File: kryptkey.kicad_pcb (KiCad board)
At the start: 2 copper layers, 30 x 36.1 mm, 36 parts, among them J1 Conn_01x04_Pin, J2 Conn_01x04_Pin, J3 USB4155-03-C_REVA, SW1 SW_Push, SW2 SW_Push, SW3 SW_Push, SW4 SW_SPDT, U1 AMS1117-3.3, U2 STM32F103C8T6, Y1 16MHz

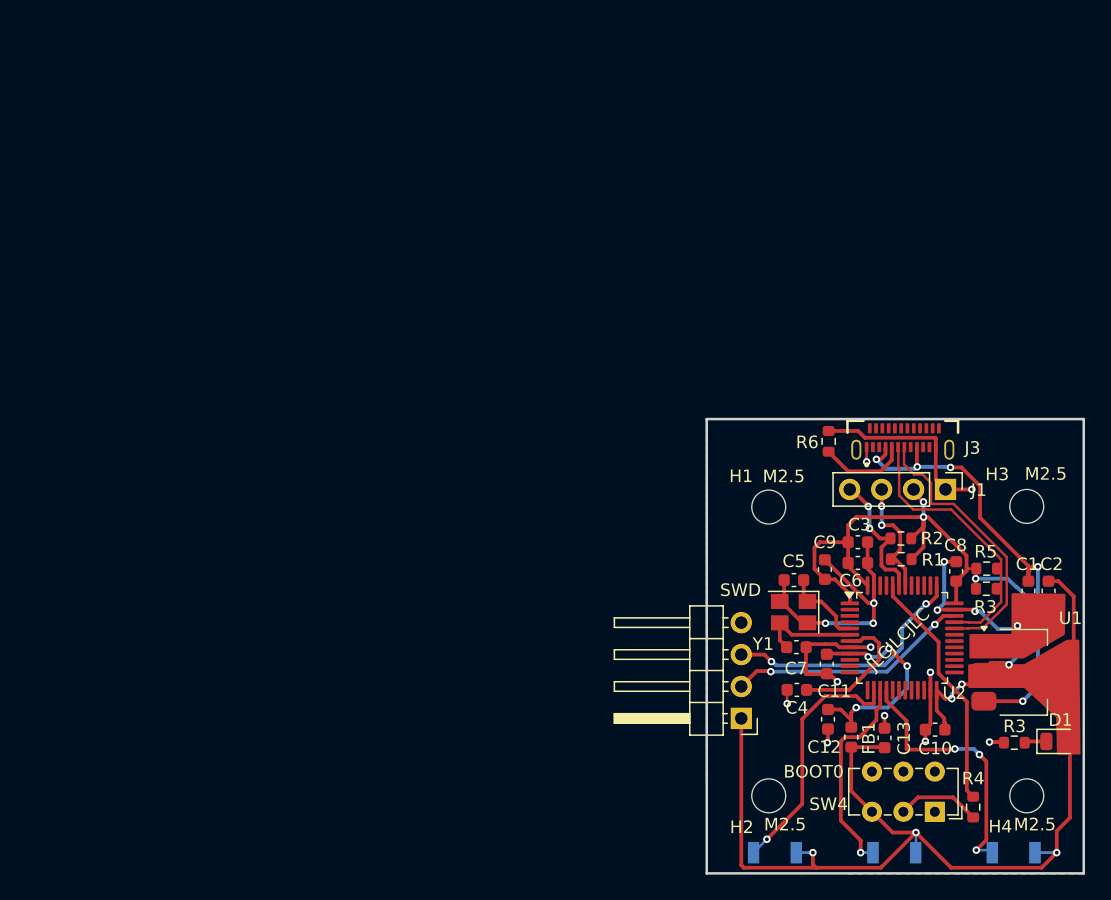
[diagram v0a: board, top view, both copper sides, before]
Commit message: v0.1 jlcpcb production order
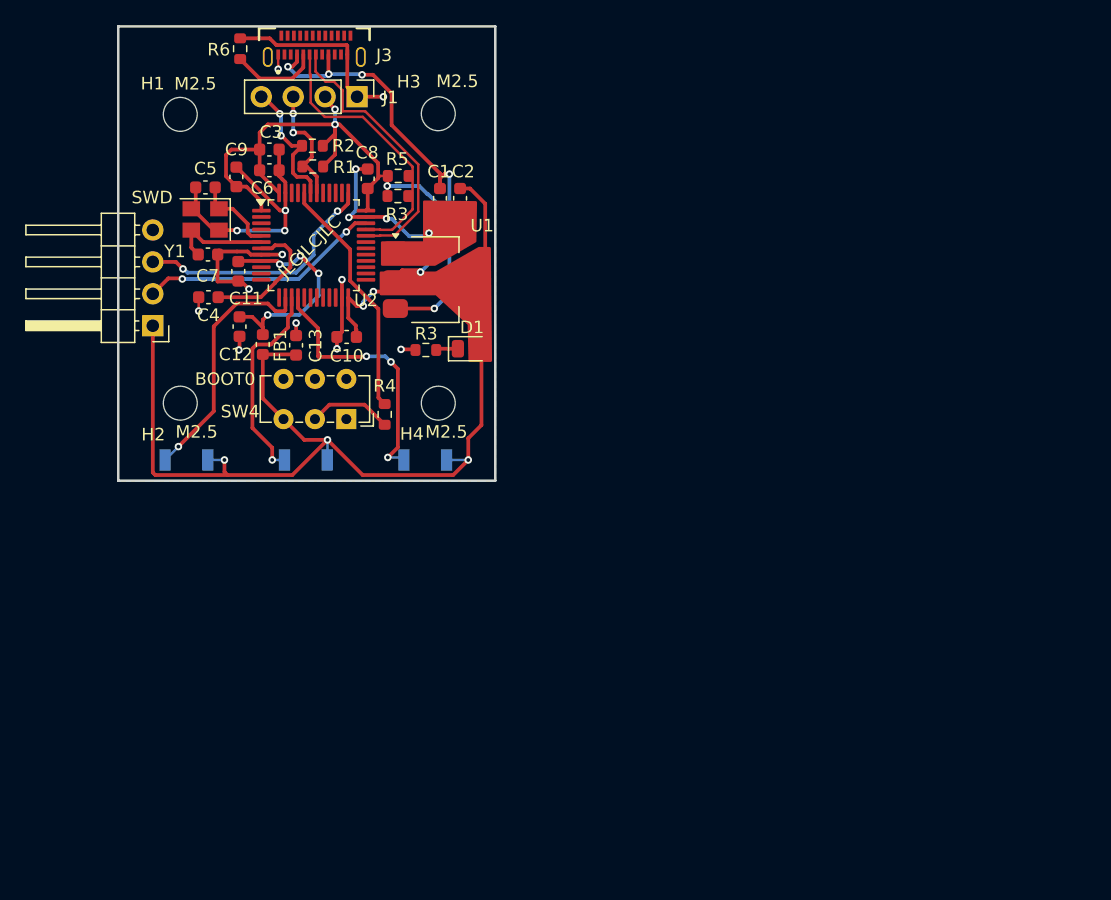
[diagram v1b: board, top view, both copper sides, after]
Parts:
- moved C1 56.3 mm to (118.7, 66.1)
- moved C8 56.3 mm to (113.0, 64.6)
- moved J3 56.3 mm to (108.7, 53.9)
- moved R1 56.3 mm to (108.6, 63.6)
- moved R3 56.3 mm to (117.6, 78.2)
- moved Y1 56.3 mm to (100.0, 67.8)
- moved C10 56.3 mm to (111.3, 77.2)
- moved C11 56.3 mm to (102.7, 71.9)
- moved C12 56.3 mm to (102.8, 76.3)
- moved C13 56.3 mm to (107.3, 77.8)
- moved C2 56.3 mm to (120.3, 66.1)
- moved C3 56.3 mm to (105.1, 62.3)
- moved C4 56.3 mm to (100.3, 74.0)
- moved C6 56.3 mm to (105.1, 63.9)
- moved C7 56.3 mm to (100.3, 70.6)
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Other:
- board size 30 x 36.1 mm -> 30 x 36.2 mm
